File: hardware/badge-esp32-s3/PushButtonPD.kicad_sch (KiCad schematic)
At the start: 4 parts, among them SW4 TS665CJ

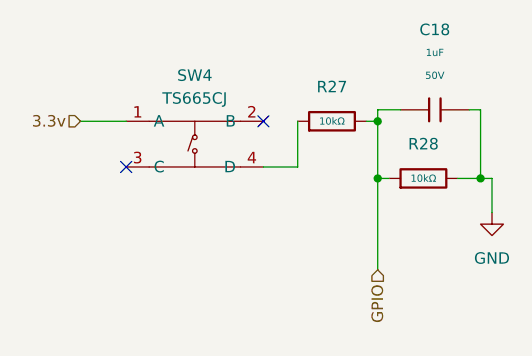
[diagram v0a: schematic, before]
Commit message: Update PushButtonPD.kicad_sch
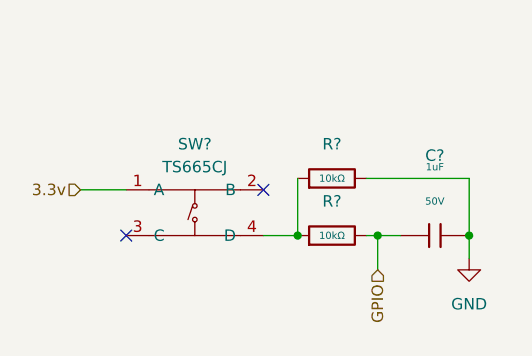
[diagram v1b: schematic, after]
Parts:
- renumbered C18 to C?, R28 to R?, R27 to R?, SW4 to SW?
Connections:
- net GND: now also R?.2; no longer R?.2
- net GPIO: now also R?.2; no longer R?.1, R?.2
- net at R?.1, SW?.4 (D): now also R?.1
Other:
- moved on the sheet: C?, R?, SW?
